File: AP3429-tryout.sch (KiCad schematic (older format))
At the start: 31 parts, among them J2 Conn_01x02, U1 AP3429, U2 AP3429, U3 AP3429, U4 AP2120N

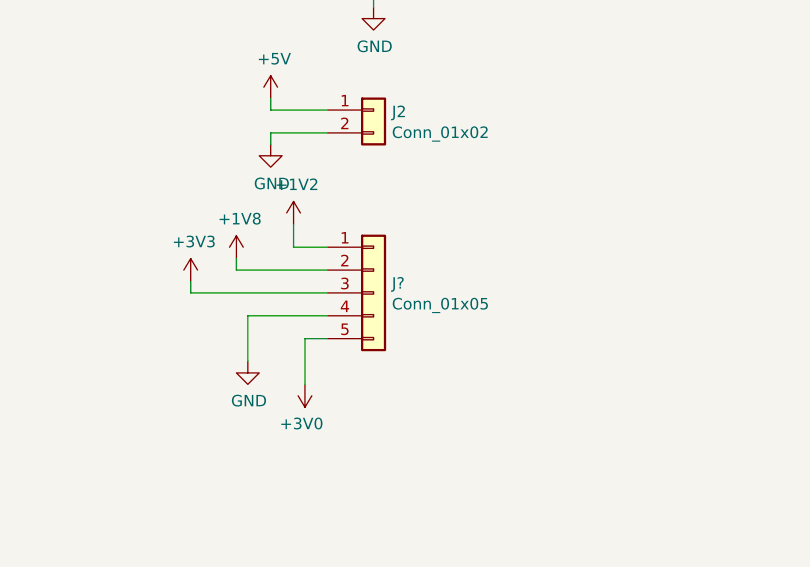
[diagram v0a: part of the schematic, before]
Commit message: update,
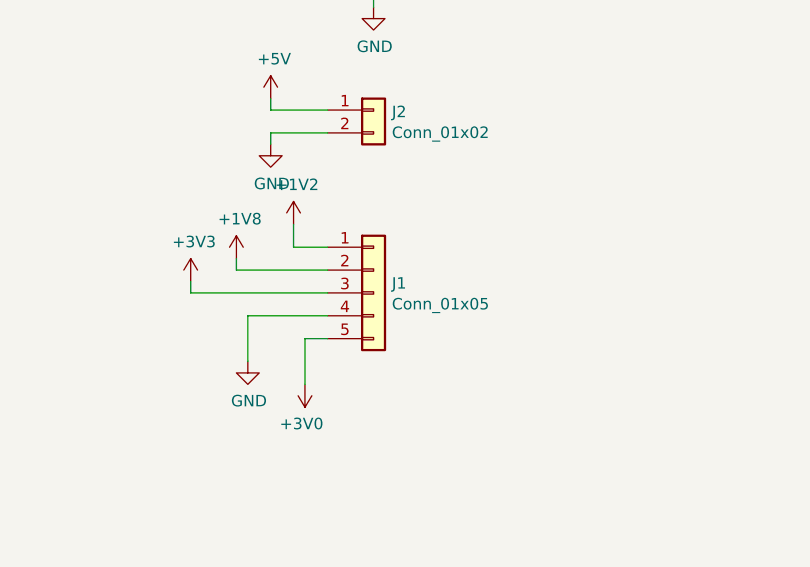
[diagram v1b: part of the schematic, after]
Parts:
- gave numbers to parts that had none: 1
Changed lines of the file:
@@
 	8550 3050 8800 3050
 $Comp
-L Connector_Generic:Conn_01x05 J?
+L Connector_Generic:Conn_01x05 J1
 U 1 1 5C04F68A
 P 9000 3850
-F 0 "J?" H 9080 3892 50  0000 L CNN
+F 0 "J1" H 9080 3892 50  0000 L CNN
 F 1 "Conn_01x05" H 9080 3801 50  0000 L CNN
 F 2 "Connector_PinHeader_2.54mm:PinHeader_1x05_P2.54mm_Vertical" H 9000 3850 50  0001 C CNN
@@
 $EndComp
 $Comp
-L my_power:+3V0 #PWR?
+L my_power:+3V0 #PWR0119
 U 1 1 5C04F76E
 P 8700 4250
-F 0 "#PWR?" H 8700 4100 50  0001 C CNN
+F 0 "#PWR0119" H 8700 4100 50  0001 C CNN
 F 1 "+3V0" H 8715 4423 50  0000 C CNN
 F 2 "" H 8700 4250 50  0001 C CNN

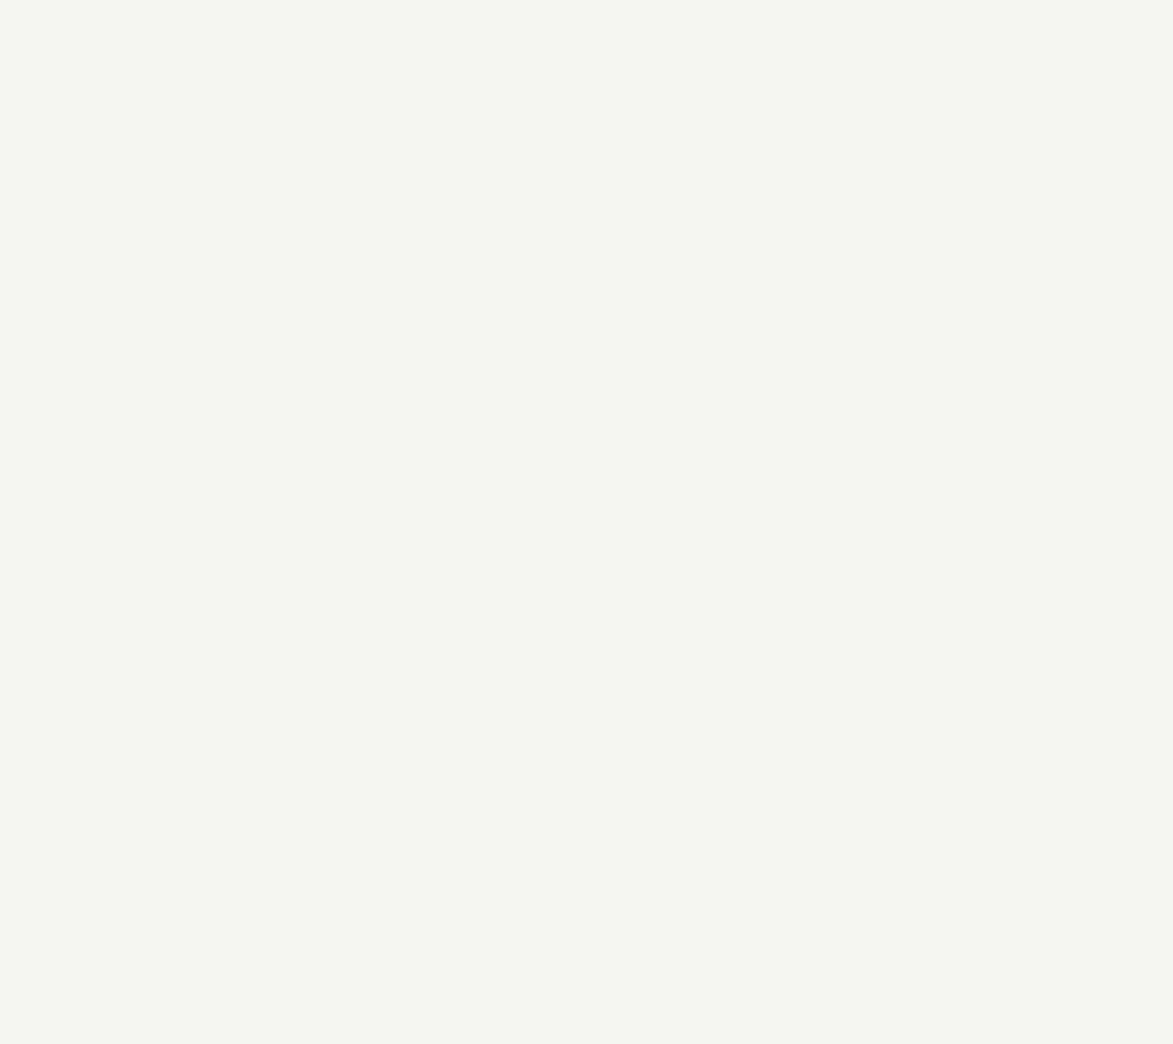
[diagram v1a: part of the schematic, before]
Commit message: update,
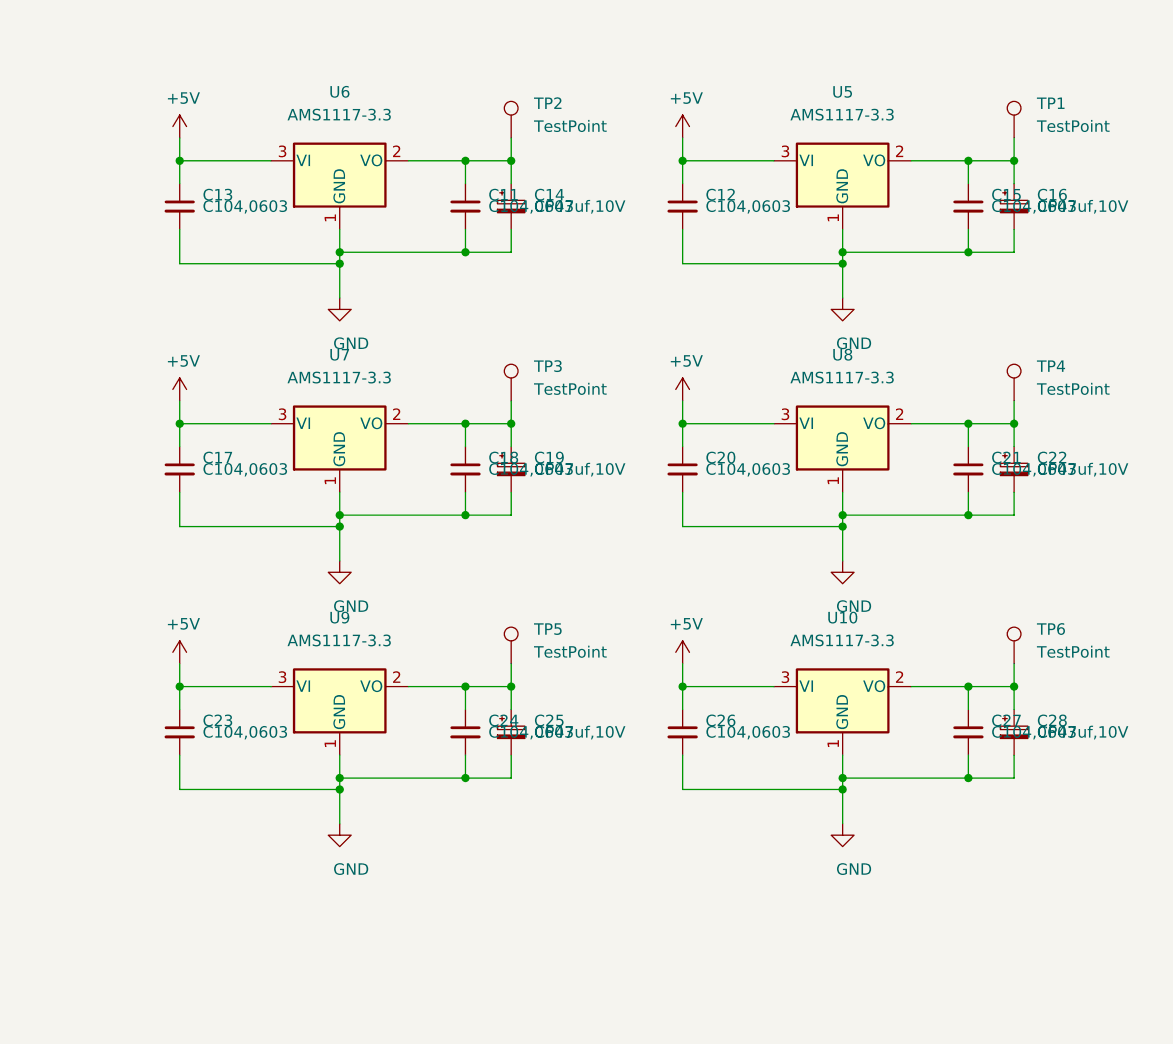
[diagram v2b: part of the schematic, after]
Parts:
- added C11, C13, C15, C17, C21, C23, C24, C26, C27: C104,0603, Capacitor_SMD:C_0603_1608Metric_Pad1.05x0.95mm_HandSolder, symbol taobao-c:C104,0603
- added C12, C18, C20: C104,0603, w_smd_cap:c_elec_5x5.3, symbol taobao-c:C104,0603
- added C14, C16, C22, C25, C28: CP47uf,10V, w_smd_cap:c_elec_5x5.3, symbol taobao-cp:CP47uf,10V
- added C19: CP47uf,10V, Capacitor_SMD:C_0603_1608Metric_Pad1.05x0.95mm_HandSolder, symbol taobao-cp:CP47uf,10V
- added TP1, TP2, TP3, TP4, TP5, TP6: TestPoint, TestPoint:TestPoint_Keystone_5019_Minature, symbol Connector:TestPoint
- added U10, U5, U6, U7, U8, U9: AMS1117-3.3, Package_TO_SOT_SMD:SOT-223-3_TabPin2, symbol Regulator_Linear:AMS1117-3.3
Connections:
- net +5V: now also C12.1, C13.1, C17.1, C20.1, C23.1, C26.1, U10.3 (VI), U5.3 (VI), U6.3 (VI), U7.3 (VI), U8.3 (VI), U9.3 (VI)
- net GND: now also C11.2, C12.2, C13.2, C14.2, C15.2, C16.2, C17.2, C18.2, C19.2, C20.2, C21.2, C22.2, C23.2, C24.2, C25.2, C26.2, C27.2, C28.2, U10.1 (GND), U5.1 (GND), U6.1 (GND), U7.1 (GND), U8.1 (GND), U9.1 (GND)
- new net: C11.1, C14.1, TP2.1, U6.2 (VO)
- new net: C18.1, C19.1, TP3.1, U7.2 (VO)
- new net: C24.1, C25.1, TP5.1, U9.2 (VO)
- new net: C15.1, C16.1, TP1.1, U5.2 (VO)
- new net: C21.1, C22.1, TP4.1, U8.2 (VO)
- new net: C27.1, C28.1, TP6.1, U10.2 (VO)

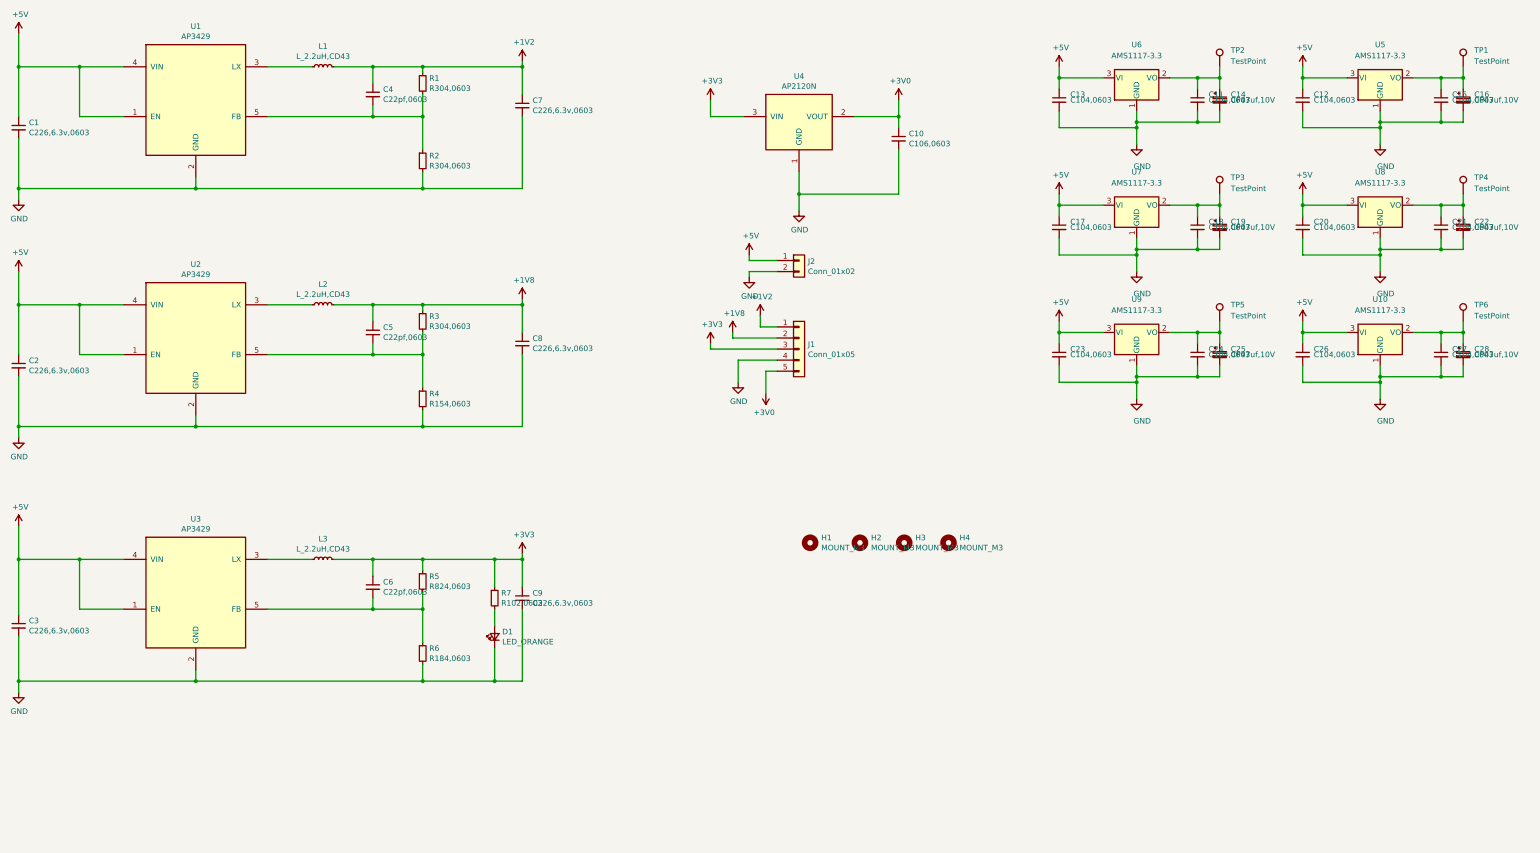
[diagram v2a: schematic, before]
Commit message: update,
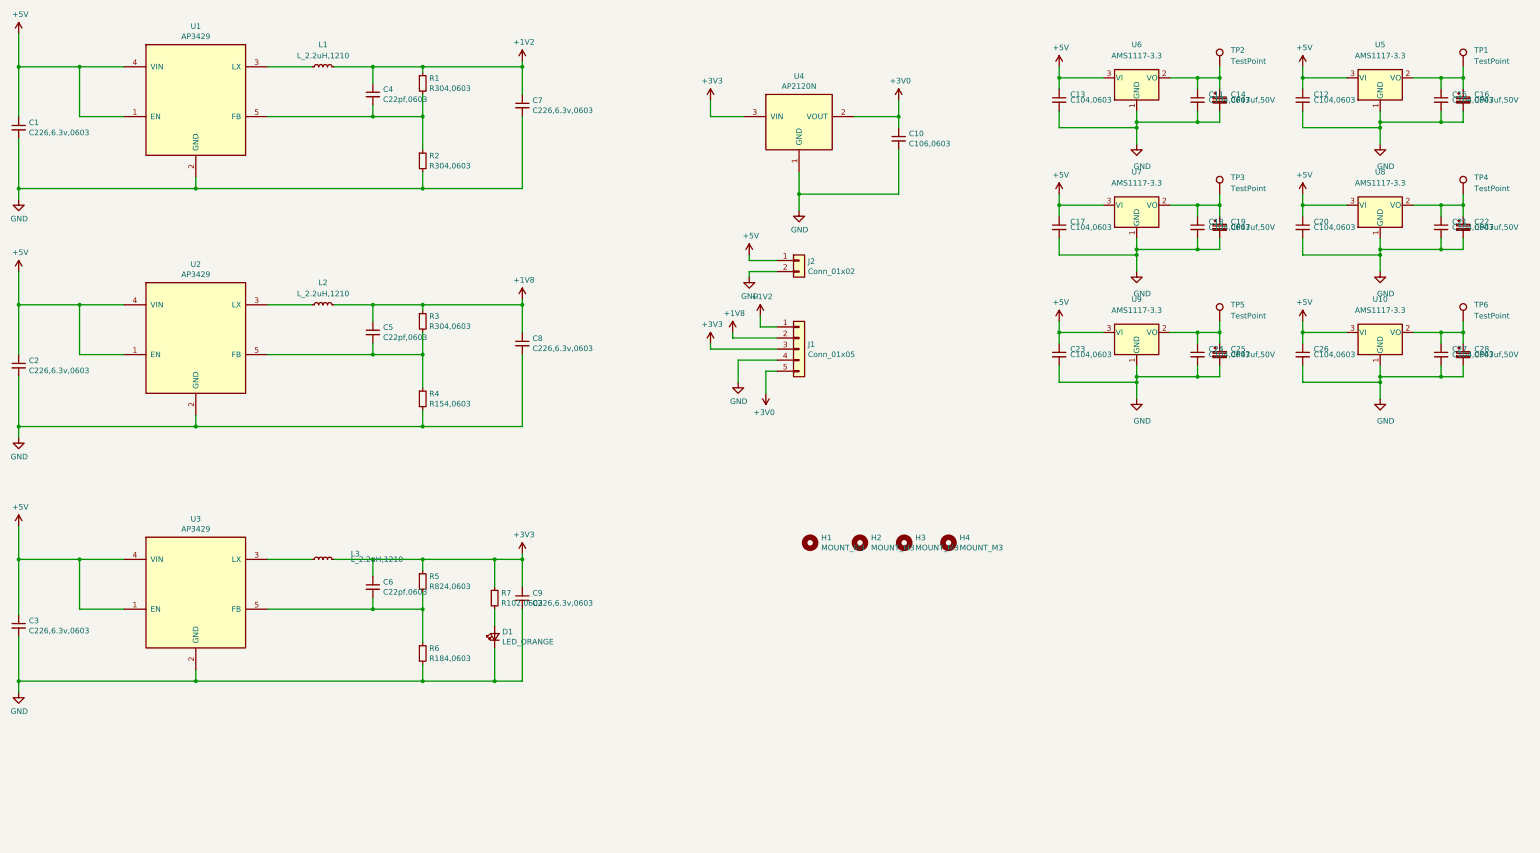
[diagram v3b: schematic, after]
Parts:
- removed C14, C16, C22, C25, C28: CP47uf,10V, w_smd_cap:c_elec_5x5.3, symbol taobao-cp:CP47uf,10V
- removed C19: CP47uf,10V, Capacitor_SMD:C_0603_1608Metric_Pad1.05x0.95mm_HandSolder, symbol taobao-cp:CP47uf,10V
- removed L1, L2, L3: L_2.2uH,CD43, w_smd_inductors:inductor_smd_4.8x2.8mm, symbol taobao-l:L_2.2uH,CD43
- added C14, C16, C19, C22, C25, C28: CP47uf,50V, w_smd_cap:c_elec_6.3x7.7, symbol taobao-cp:CP47uf,50V
- added L1, L2, L3: L_2.2uH,1210, Inductor_SMD:L_1210_3225Metric_Pad1.42x2.65mm_HandSolder, symbol taobao-l:L_2.2uH,1210
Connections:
- net +1V2: now also L1.2
- net +1V8: now also L2.2
- net +3V3: now also L3.2
- net GND: now also C14.2, C16.2, C19.2, C22.2, C25.2, C28.2
- net at U1.3 (LX): now also L1.1
- net at U2.3 (LX): now also L2.1
- net at U3.3 (LX): now also L3.1
- net at C11.1, TP2.1, U6.2 (VO): now also C14.1
- net at C18.1, TP3.1, U7.2 (VO): now also C19.1
- net at C24.1, TP5.1, U9.2 (VO): now also C25.1
- net at C15.1, TP1.1, U5.2 (VO): now also C16.1
- net at C21.1, TP4.1, U8.2 (VO): now also C22.1
- net at C27.1, TP6.1, U10.2 (VO): now also C28.1
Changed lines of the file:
@@
-$EndComp
-$Comp
-L taobao-l:L_2.2uH,CD43 L1
-U 1 1 5C06343C
-P 4700 1300
-F 0 "L1" V 4885 1300 50  0000 C CNN
-F 1 "L_2.2uH,CD43" V 4794 1300 50  0000 C CNN
-F 2 "w_smd_inductors:inductor_smd_4.8x2.8mm" H 4700 1300 50  0001 C CNN
-F 3 "" H 4700 1300 50  0001 C CNN
-	1    4700 1300
-	0    -1   -1   0
-$EndComp
-$Comp
-L taobao-l:L_2.2uH,CD43 L2
-U 1 1 5C063614
-P 4700 3450
-F 0 "L2" V 4885 3450 50  0000 C CNN
-F 1 "L_2.2uH,CD43" V 4794 3450 50  0000 C CNN
-F 2 "w_smd_inductors:inductor_smd_4.8x2.8mm" H 4700 3450 50  0001 C CNN
-F 3 "" H 4700 3450 50  0001 C CNN
-	1    4700 3450
-	0    -1   -1   0
-$EndComp
-$Comp
-L taobao-l:L_2.2uH,CD43 L3
-U 1 1 5C0638E1
-P 4700 5750
-F 0 "L3" V 4885 5750 50  0000 C CNN
-F 1 "L_2.2uH,CD43" V 4794 5750 50  0000 C CNN
-F 2 "w_smd_inductors:inductor_smd_4.8x2.8mm" H 4700 5750 50  0001 C CNN
-F 3 "" H 4700 5750 50  0001 C CNN
-	1    4700 5750
-	0    -1   -1   0
 $EndComp
 $Comp
@@
 $EndComp
 $Comp
-L taobao-cp:CP47uf,10V C14
-U 1 1 5C050395
-P 12800 1600
-F 0 "C14" H 12900 1650 50  0000 L CNN
-F 1 "CP47uf,10V" H 12900 1600 50  0000 L CNN
-F 2 "w_smd_cap:c_elec_5x5.3" H 12800 1600 50  0001 C CNN
-F 3 "~" H 12800 1600 50  0001 C CNN
-	1    12800 1600
-	1    0    0    -1
-$EndComp
-$Comp
 L power:GND #PWR0120
 U 1 1 5C050571
@@
 $EndComp
 $Comp
-L taobao-cp:CP47uf,10V C19
-U 1 1 5C0A360B
-P 12800 2750
-F 0 "C19" H 12900 2800 50  0000 L CNN
-F 1 "CP47uf,10V" H 12900 2750 50  0000 L CNN
-F 2 "Capacitor_SMD:C_0603_1608Metric_Pad1.05x0.95mm_HandSolder" H 12800 2750 50  0001 C CNN
-F 3 "~" H 12800 2750 50  0001 C CNN
-	1    12800 2750
-	1    0    0    -1
-$EndComp
-$Comp
 L power:GND #PWR0122
 U 1 1 5C0A3611
@@
 $EndComp
 $Comp
-L taobao-cp:CP47uf,10V C25
-U 1 1 5C0A7CEB
-P 12800 3900
-F 0 "C25" H 12900 3950 50  0000 L CNN
-F 1 "CP47uf,10V" H 12900 3900 50  0000 L CNN
-F 2 "w_smd_cap:c_elec_5x5.3" H 12800 3900 50  0001 C CNN
-F 3 "~" H 12800 3900 50  0001 C CNN
-	1    12800 3900
-	1    0    0    -1
-$EndComp
-$Comp
 L power:GND #PWR0124
 U 1 1 5C0A7CF1
@@
 $EndComp
 $Comp
-L taobao-cp:CP47uf,10V C16
-U 1 1 5C0AD753
-P 15000 1600
-F 0 "C16" H 15100 1650 50  0000 L CNN
-F 1 "CP47uf,10V" H 15100 1600 50  0000 L CNN
-F 2 "w_smd_cap:c_elec_5x5.3" H 15000 1600 50  0001 C CNN
-F 3 "~" H 15000 1600 50  0001 C CNN
-	1    15000 1600
-	1    0    0    -1
-$EndComp
-$Comp
 L power:GND #PWR0126
 U 1 1 5C0AD759
@@
 $EndComp
 $Comp
-L taobao-cp:CP47uf,10V C22
-U 1 1 5C0AD794
-P 15000 2750
-F 0 "C22" H 15100 2800 50  0000 L CNN
-F 1 "CP47uf,10V" H 15100 2750 50  0000 L CNN
-F 2 "w_smd_cap:c_elec_5x5.3" H 15000 2750 50  0001 C CNN
-F 3 "~" H 15000 2750 50  0001 C CNN
-	1    15000 2750
-	1    0    0    -1
-$EndComp
-$Comp
 L power:GND #PWR0128
 U 1 1 5C0AD79A
@@
 $EndComp
 $Comp
-L taobao-cp:CP47uf,10V C28
-U 1 1 5C0AD7D5
-P 15000 3900
-F 0 "C28" H 15100 3950 50  0000 L CNN
-F 1 "CP47uf,10V" H 15100 3900 50  0000 L CNN
-F 2 "w_smd_cap:c_elec_5x5.3" H 15000 3900 50  0001 C CNN
-F 3 "~" H 15000 3900 50  0001 C CNN
-	1    15000 3900
-	1    0    0    -1
-$EndComp
-$Comp
 L power:GND #PWR0130
 U 1 1 5C0AD7DB
@@
 Wire Wire Line
 	14800 4100 15000 4100
+$Comp
+L taobao-cp:CP47uf,50V C14
+U 1 1 5C04F10F
+P 12800 1600
+F 0 "C14" H 12900 1650 50  0000 L CNN
+F 1 "CP47uf,50V" H 12900 1600 50  0000 L CNN
+F 2 "w_smd_cap:c_elec_6.3x7.7" H 12800 1600 50  0001 C CNN
+F 3 "~" H 12800 1600 50  0001 C CNN
+	1    12800 1600
+	1    0    0    -1
+$EndComp
+$Comp
+L taobao-cp:CP47uf,50V C16
+U 1 1 5C04F461
+P 15000 1600
+F 0 "C16" H 15100 1650 50  0000 L CNN
+F 1 "CP47uf,50V" H 15100 1600 50  0000 L CNN
+F 2 "w_smd_cap:c_elec_6.3x7.7" H 15000 1600 50  0001 C CNN
+F 3 "~" H 15000 1600 50  0001 C CNN
+	1    15000 1600
+	1    0    0    -1
+$EndComp
+$Comp
+L taobao-cp:CP47uf,50V C19
+U 1 1 5C062EA4
+P 12800 2750
+F 0 "C19" H 12900 2800 50  0000 L CNN
+F 1 "CP47uf,50V" H 12900 2750 50  0000 L CNN
+F 2 "w_smd_cap:c_elec_6.3x7.7" H 12800 2750 50  0001 C CNN
+F 3 "~" H 12800 2750 50  0001 C CNN
+	1    12800 2750
+	1    0    0    -1
+$EndComp
+$Comp
+L taobao-cp:CP47uf,50V C22
+U 1 1 5C062F52
+P 15000 2750
+F 0 "C22" H 15100 2800 50  0000 L CNN
+F 1 "CP47uf,50V" H 15100 2750 50  0000 L CNN
+F 2 "w_smd_cap:c_elec_6.3x7.7" H 15000 2750 50  0001 C CNN
+F 3 "~" H 15000 2750 50  0001 C CNN
+	1    15000 2750
+	1    0    0    -1
+$EndComp
+$Comp
+L taobao-cp:CP47uf,50V C25
+U 1 1 5C063012
+P 12800 3900
+F 0 "C25" H 12900 3950 50  0000 L CNN
+F 1 "CP47uf,50V" H 12900 3900 50  0000 L CNN
+F 2 "w_smd_cap:c_elec_6.3x7.7" H 12800 3900 50  0001 C CNN
+F 3 "~" H 12800 3900 50  0001 C CNN
+	1    12800 3900
+	1    0    0    -1
+$EndComp
+$Comp
+L taobao-cp:CP47uf,50V C28
+U 1 1 5C0630F4
+P 15000 3900
+F 0 "C28" H 15100 3950 50  0000 L CNN
+F 1 "CP47uf,50V" H 15100 3900 50  0000 L CNN
+F 2 "w_smd_cap:c_elec_6.3x7.7" H 15000 3900 50  0001 C CNN
+F 3 "~" H 15000 3900 50  0001 C CNN
+	1    15000 3900
+	1    0    0    -1
+$EndComp
+$Comp
+L taobao-l:L_2.2uH,1210 L1
+U 1 1 5C0651A2
+P 4700 1300
+F 0 "L1" V 4900 1300 50  0000 C CNN
+F 1 "L_2.2uH,1210" V 4800 1300 50  0000 C CNN
+F 2 "Inductor_SMD:L_1210_3225Metric_Pad1.42x2.65mm_HandSolder" H 4700 1300 50  0001 C CNN
+F 3 "" H 4700 1300 50  0001 C CNN
+	1    4700 1300
+	0    -1   -1   0
+$EndComp
+$Comp
+L taobao-l:L_2.2uH,1210 L2
+U 1 1 5C0652FE
+P 4700 3450
+F 0 "L2" V 4900 3450 50  0000 C CNN
+F 1 "L_2.2uH,1210" V 4800 3450 50  0000 C CNN
+F 2 "Inductor_SMD:L_1210_3225Metric_Pad1.42x2.65mm_HandSolder" H 4700 3450 50  0001 C CNN
+F 3 "" H 4700 3450 50  0001 C CNN
+	1    4700 3450
+	0    -1   -1   0
+$EndComp
+$Comp
+L taobao-l:L_2.2uH,1210 L3
+U 1 1 5C0655CA
+P 4700 5750
+F 0 "L3" V 4750 5500 50  0000 R CNN
+F 1 "L_2.2uH,1210" V 4700 5500 50  0000 R CNN
+F 2 "Inductor_SMD:L_1210_3225Metric_Pad1.42x2.65mm_HandSolder" H 4700 5750 50  0001 C CNN
+F 3 "" H 4700 5750 50  0001 C CNN
+	1    4700 5750
+	0    -1   -1   0
+$EndComp
 $EndSCHEMATC

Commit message: update,
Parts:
- C12, C18, C20: footprint w_smd_cap:c_elec_5x5.3 -> Capacitor_SMD:C_0603_1608Metric_Pad1.05x0.95mm_HandSolder
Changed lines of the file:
@@
 F 0 "C18" H 12700 2800 50  0000 L CNN
 F 1 "C104,0603" H 12700 2750 50  0000 L CNN
-F 2 "w_smd_cap:c_elec_5x5.3" H 12600 2750 50  0001 C CNN
+F 2 "Capacitor_SMD:C_0603_1608Metric_Pad1.05x0.95mm_HandSolder" H 12600 2750 50  0001 C CNN
 F 3 "~" H 12600 2750 50  0001 C CNN
 	1    12600 2750
@@
 F 0 "C12" H 13650 1650 50  0000 L CNN
 F 1 "C104,0603" H 13650 1600 50  0000 L CNN
-F 2 "w_smd_cap:c_elec_5x5.3" H 13550 1600 50  0001 C CNN
+F 2 "Capacitor_SMD:C_0603_1608Metric_Pad1.05x0.95mm_HandSolder" H 13550 1600 50  0001 C CNN
 F 3 "~" H 13550 1600 50  0001 C CNN
 	1    13550 1600
@@
 F 0 "C20" H 13650 2800 50  0000 L CNN
 F 1 "C104,0603" H 13650 2750 50  0000 L CNN
-F 2 "w_smd_cap:c_elec_5x5.3" H 13550 2750 50  0001 C CNN
+F 2 "Capacitor_SMD:C_0603_1608Metric_Pad1.05x0.95mm_HandSolder" H 13550 2750 50  0001 C CNN
 F 3 "~" H 13550 2750 50  0001 C CNN
 	1    13550 2750
